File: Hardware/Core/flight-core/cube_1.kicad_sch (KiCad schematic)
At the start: 19 parts, among them J10 Conn_02x06_Counter_Clockwise, J11 Conn_01x04_Socket, J12 Conn_01x04_Socket, J13 MicroFit_VT_3, J8 MicroFit_VT_3, J9 Cube Orange Plus Female Header, Q1 MMBF170, Q2 MMBF170, Q3 MMBF170

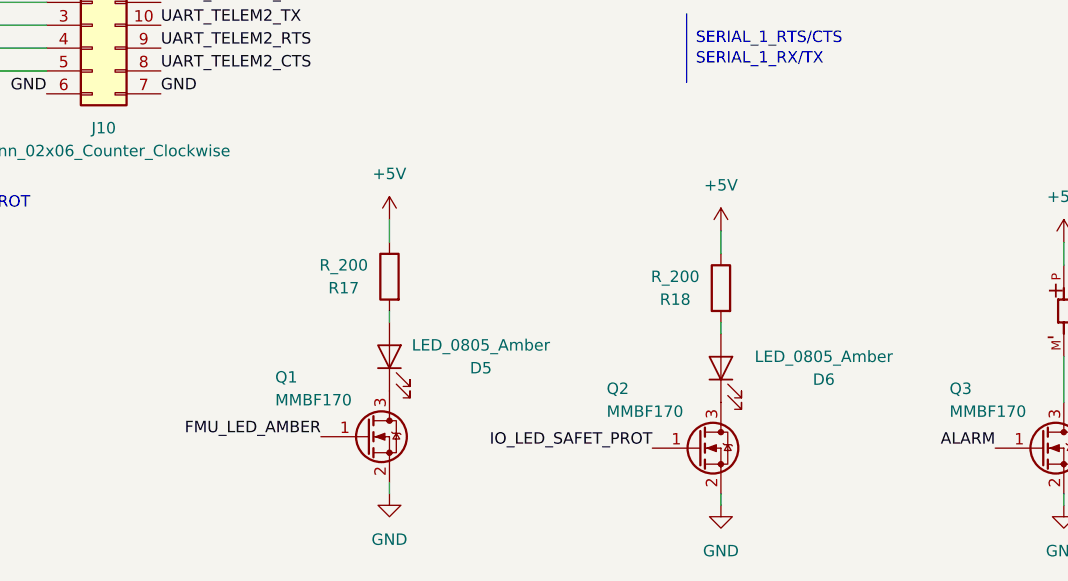
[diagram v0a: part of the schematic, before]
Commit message: updating mini tps to new symbol and footprint
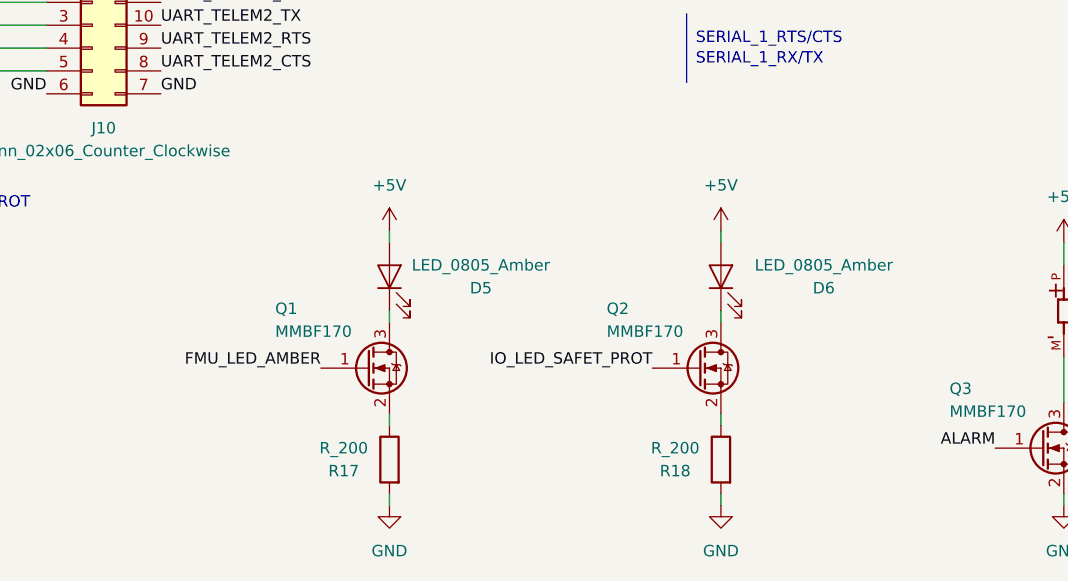
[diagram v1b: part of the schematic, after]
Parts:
- TP10, TP7, TP8, TP9: footprint TestPoint:TestPoint_Pad_D1.0mm -> obad_footprints:TestPoint_Pad_D1.0mm
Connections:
- net +5V: now also D5.2 (A), D6.2 (A); no longer R17.1, R18.1
- net GND: now also R17.2, R18.2; no longer Q1.2 (S), Q2.2 (S)
- new net: Q2.2 (S), R18.1
- new net: Q1.2 (S), R17.1
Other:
- moved on the sheet: D5, D6, Q1, Q2, R17, R18
